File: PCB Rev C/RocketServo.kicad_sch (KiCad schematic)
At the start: 33 parts, among them IC1 PIC12F1822-I/SN, P1 Conn_01x02, P2 Conn_01x03, P3 Conn_01x02, SW1 SW_Push, SW2 SW_Push, U1 L7806, U2 L78L05_SOT89, U3 CPC1017N, U4 CPC1017N

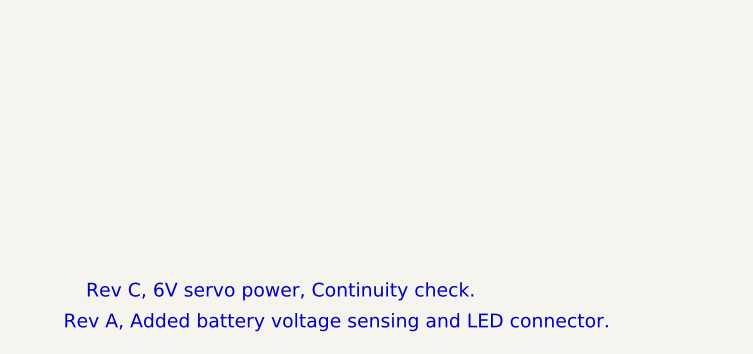
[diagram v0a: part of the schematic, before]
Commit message: Rev C1
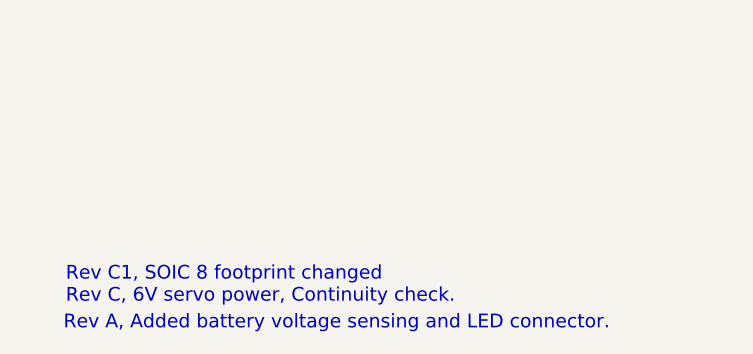
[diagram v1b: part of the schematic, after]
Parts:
- IC1: footprint Package_SO:SOIC-8_5.23x5.23mm_P1.27mm -> Package_SO:SOIC-8_3.9x4.9mm_P1.27mm
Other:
- note added: "Rev C1, SOIC 8 footprint changed Rev C, 6V servo power, Continuity check."
- note removed: "Rev C, 6V servo power, Continuity check."
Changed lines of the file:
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@@
 		(title "Rocket Servo")
 		(date "2024-09-23")
-		(rev "C")
+		(rev "C1")
 		(company "DMFE")
 		(comment 1 "Altimeter triggered servo")
@@
 		)
 	)
-	(text "Rev C, 6V servo power, Continuity check."
+	(text "Rev C1, SOIC 8 footprint changed\nRev C, 6V servo power, Continuity check."
 		(exclude_from_sim no)
-		(at 49.53 189.992 0)
+		(at 25.654 189.23 0)
 		(effects
 			(font
 				(size 1.524 1.524)
 			)
+			(justify left)
 		)
 	)
@@
 			)
 		)
-		(property "Footprint" "Package_SO:SOIC-8_5.23x5.23mm_P1.27mm"
+		(property "Footprint" "Package_SO:SOIC-8_3.9x4.9mm_P1.27mm"
 			(at 110.49 124.46 0)
 			(effects
